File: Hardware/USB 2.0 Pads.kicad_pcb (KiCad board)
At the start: 2 copper layers, 26 x 14 mm, 5 parts, among them J1 USB_A, P1 USB_C_Plug_USB2.0

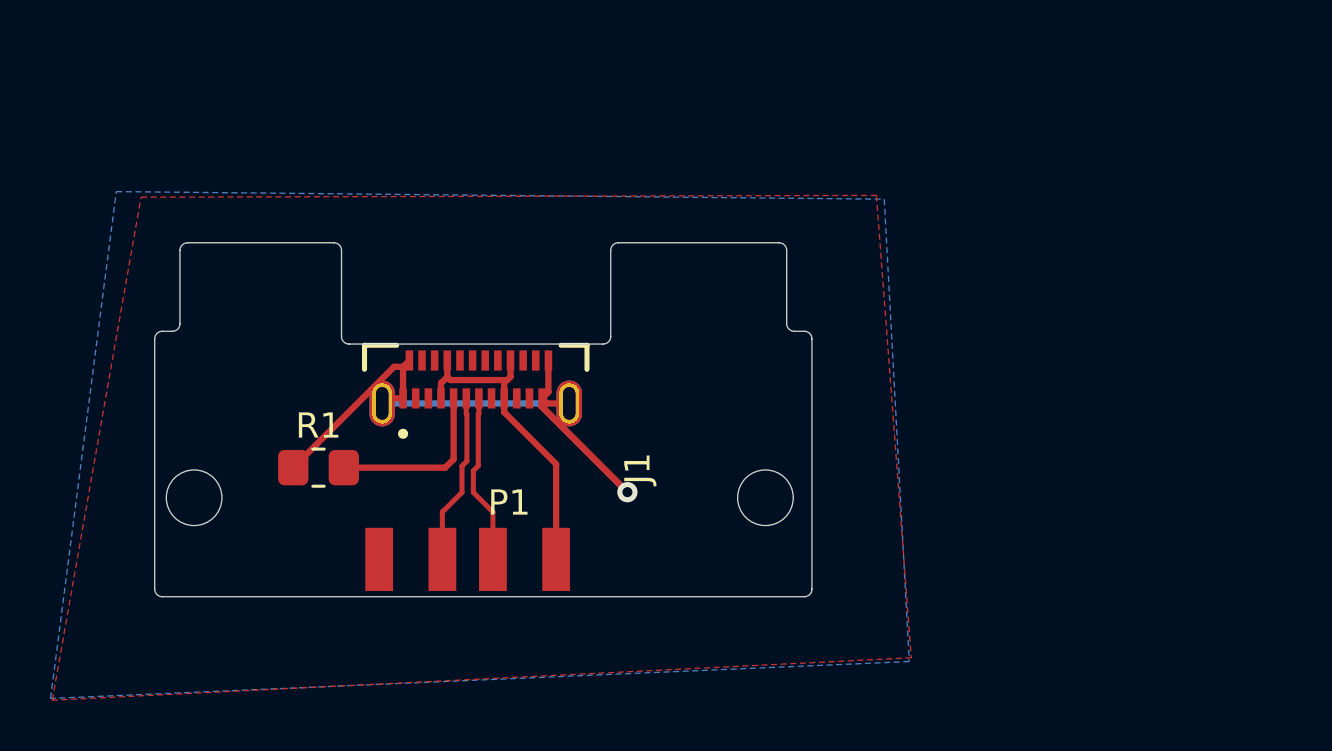
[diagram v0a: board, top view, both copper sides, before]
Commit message: Updated files
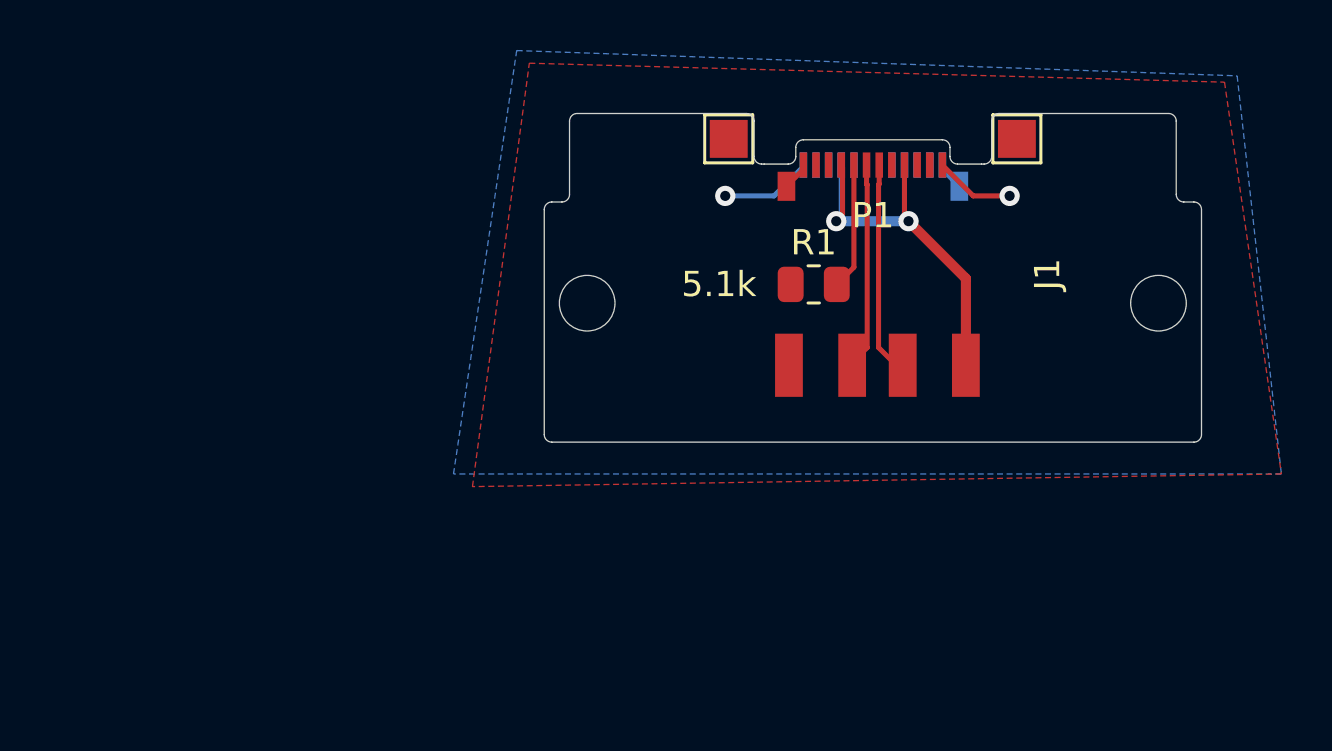
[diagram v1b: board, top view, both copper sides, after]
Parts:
- added TP1: TestPoint, TestPoint:TestPoint_Pad_1.5x1.5mm, F.Cu at (175.4, 89.2)
- added TP3: TestPoint, TestPoint:TestPoint_Pad_1.5x1.5mm, F.Cu at (186.8, 89.2)
- H1: value (none) -> MountingHole
- P1: footprint SnapEDA Library:GCT_USB4155-03-C_REVA -> Expansion_Card:USB_C_Plug_Molex_105444
- R1: footprint Resistor_SMD:R_0805_2012Metric_Pad1.20x1.40mm_HandSolder -> Resistor_SMD:R_0805_2012Metric
- moved R1 20.9 mm to (178.8, 95.0)
- moved J1 17.9 mm to (180.0, 101.5)
- moved P1 17.9 mm to (181.1, 90.2), turned to 0 degrees
- moved H1 17.3 mm to (169.8, 95.7)
- moved H2 17.3 mm to (192.4, 95.7)
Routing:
- net Net-(J1-Pad4): track 27.5 -> 9.03 mm, vias 1 -> 2
- net Net-(J1-Pad1): track 12.8 -> 18.7 mm, vias 0 -> 2
- net Net-(P1-PadA5): track 6.89 -> 5.00 mm
- net D-: track 6.78 -> 8.58 mm
- net D+: track 6.78 -> 8.07 mm
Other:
- board size 26 x 14 mm -> 26 x 13 mm
